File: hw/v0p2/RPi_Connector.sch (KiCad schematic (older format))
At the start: 1 part, among them P1 Conn_02x20_Odd_Even

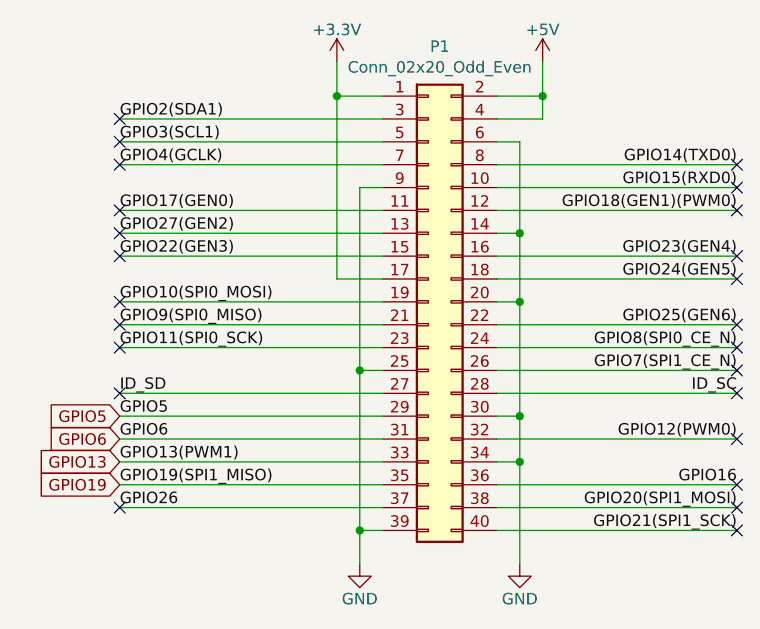
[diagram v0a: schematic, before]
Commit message: Updated
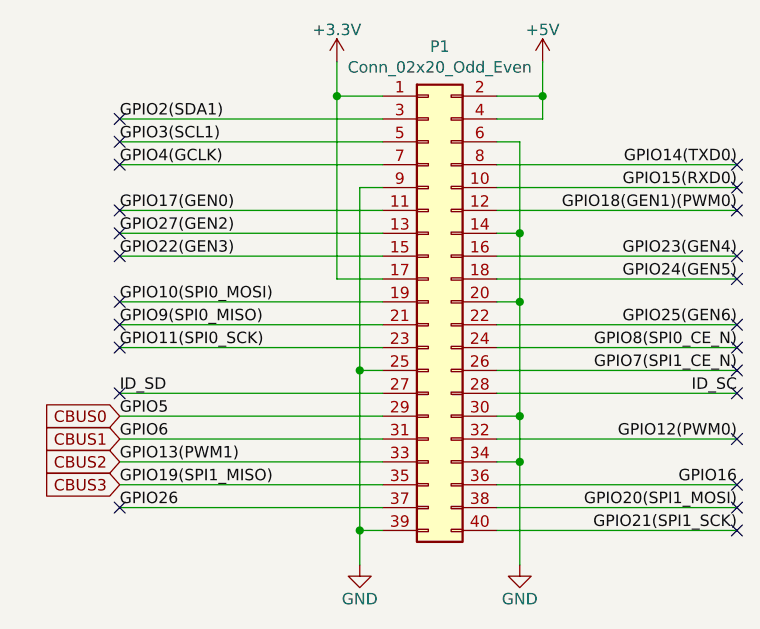
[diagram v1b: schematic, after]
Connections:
- net GPIO13 renamed CBUS2
- net GPIO19 renamed CBUS3
- net GPIO5 renamed CBUS0
- net GPIO6 renamed CBUS1
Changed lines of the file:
@@
 $Descr A4 11693 8268
 encoding utf-8
-Sheet 2 3
+Sheet 2 5
 Title ""
 Date ""
@@
 Wire Wire Line
 	3250 2000 3250 2300
-Text GLabel 1500 3000 0    50   Input ~ 0
-GPIO13
-Text GLabel 1500 3100 0    50   Input ~ 0
-GPIO19
-Text GLabel 1500 2900 0    50   Input ~ 0
-GPIO6
-Text GLabel 1500 2800 0    50   Input ~ 0
-GPIO5
 NoConn ~ 1500 3200
 NoConn ~ 1500 2700
@@
 NoConn ~ 4200 3200
 NoConn ~ 4200 3300
+Text GLabel 1500 3100 0    50   Input ~ 0
+CBUS3
+Text GLabel 1500 3000 0    50   Input ~ 0
+CBUS2
+Text GLabel 1500 2900 0    50   Input ~ 0
+CBUS1
+Text GLabel 1500 2800 0    50   Input ~ 0
+CBUS0
 $EndSCHEMATC
